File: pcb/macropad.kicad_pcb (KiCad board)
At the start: 2 copper layers, 90 x 67 mm, 26 parts, among them J1 OLED_DISPLAY, SW1 SW_Push, SW2 SW_Push, SW3 SW_Push, SW4 SW_Push, SW5 RotaryEncoder_Switch, SW6 SW_Push, SW7 SW_Push, U1 Seeed Studio XIAO RP2040

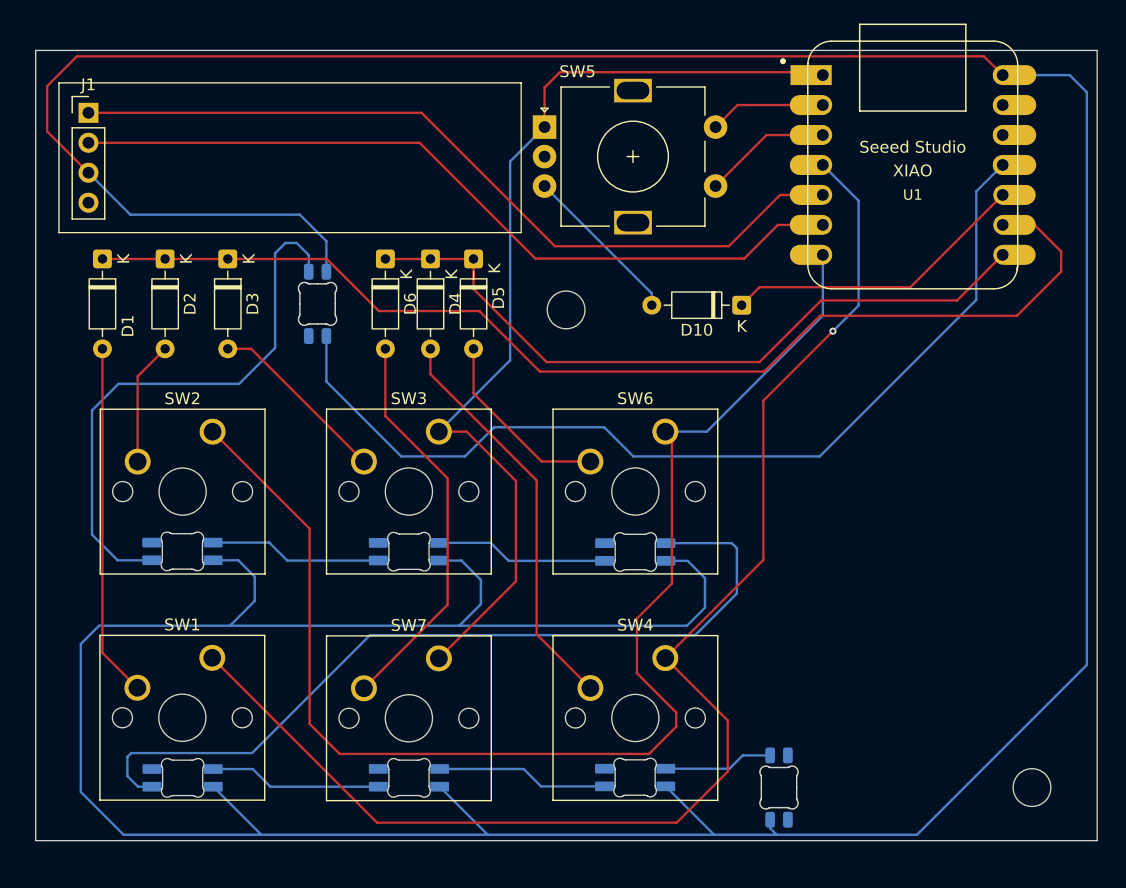
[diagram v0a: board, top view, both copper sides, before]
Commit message: V1.4 - Reworked GND fields, solved all errors, added Steve
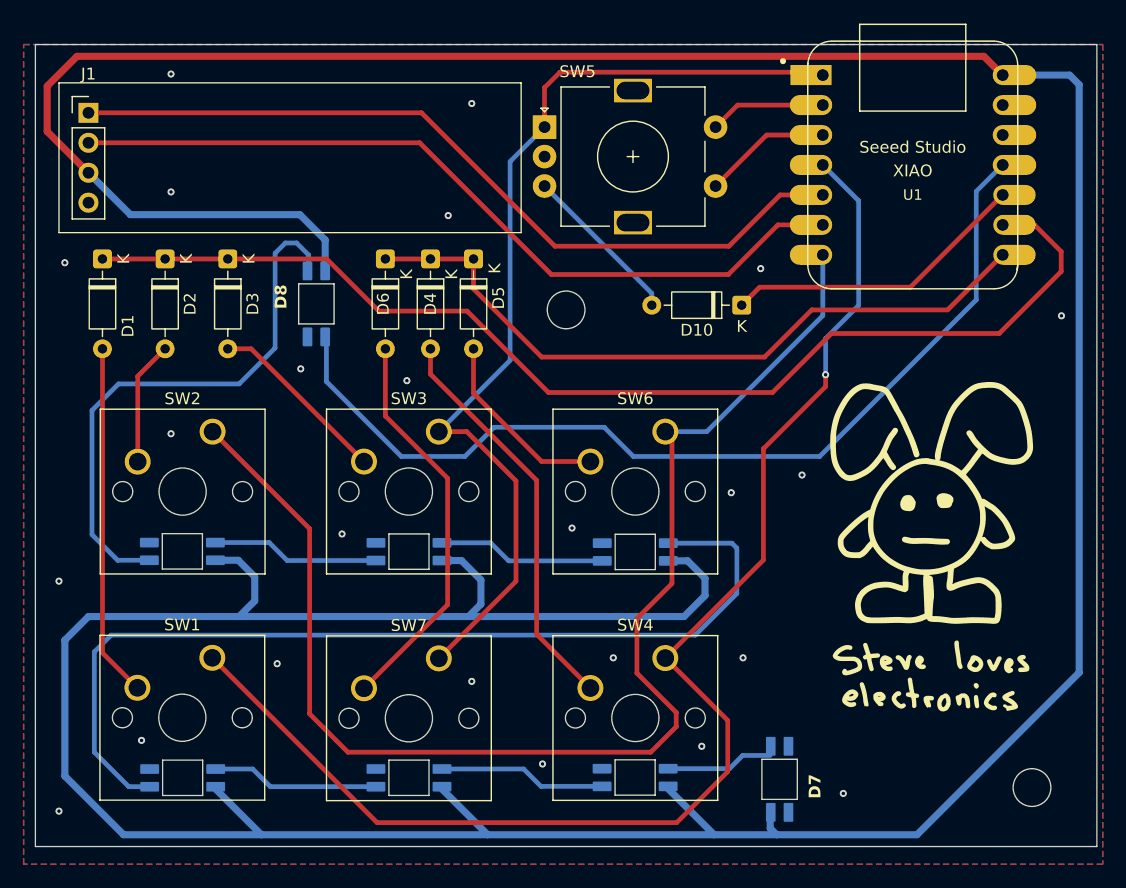
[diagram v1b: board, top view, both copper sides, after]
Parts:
- D11, D12, D13, D14, D15, D9: footprint Cherry-MX:MX_SK6812MINI-E -> Libraries:MX_SK6812MINI-E
- D7, D8: footprint LED_SMD:LED_SK6812MINI-E_3.2x2.8mm_P1.5mm_ReverseMount -> Libraries:SK6812MINI-E_fixed; moved to F.Cu
- U1: footprint Hackpad:XIAO-Generic-Hybrid-14P-2.54-21X17.8MM -> Libraries:XIAO-Generic-Hybrid-14P-2.54-21X17.8MM
- moved D7 0.70 mm to (170.5, 104.8)
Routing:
- net Net-(D12-DOUT): track 71.5 -> 81.2 mm
- net Row 1: track 96.3 -> 97.8 mm
- net VCC: track 375.7 -> 374.5 mm
- net SCL: track 67.5 -> 68.6 mm
- net Column 2: track 111.7 -> 111.1 mm
- net GND: vias 0 -> 24
- added copper zone on B.Cu, net GND
- added copper zone on F.Cu, net GND
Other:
- board size 90 x 67 mm -> 90 x 68 mm
